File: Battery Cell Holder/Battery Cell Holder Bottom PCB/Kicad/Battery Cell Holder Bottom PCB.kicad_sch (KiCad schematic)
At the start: 10 parts

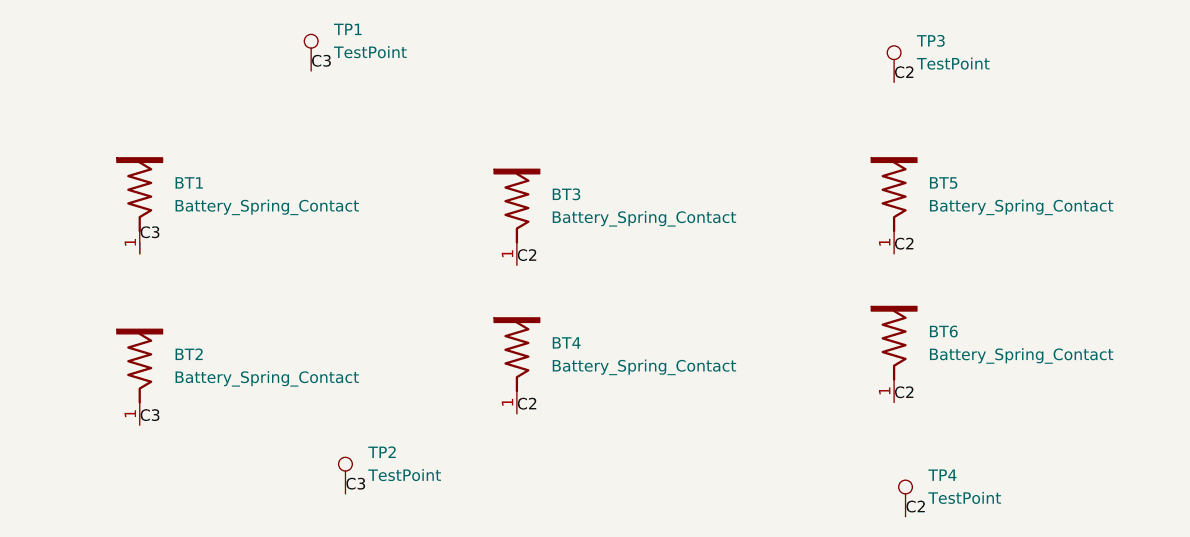
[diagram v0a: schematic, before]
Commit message: fixes to boards
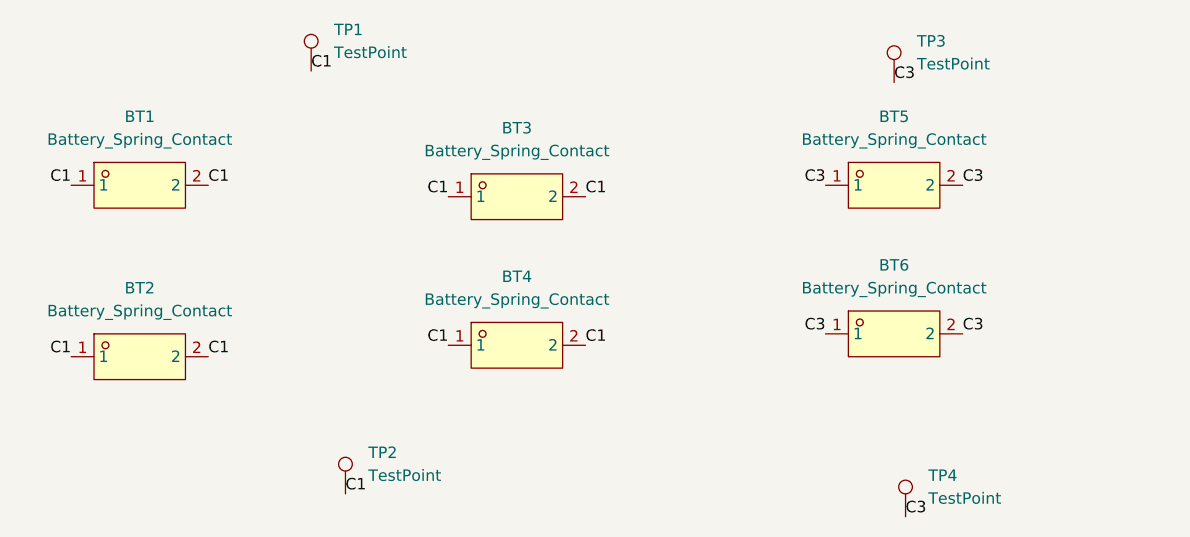
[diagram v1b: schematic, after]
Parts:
- BT1, BT2, BT3, BT4, BT5, BT6: footprint BatterySpringContact:Keystone_5222_SpringContact_THM -> C19724688:TH-2_BD10.0_F10-12-0.5-1.3UU-SUS304; symbol BatterySpringContact:Battery_Spring_Contact -> C19724688:F10-12-0.5-1.3UU-SUS304; LCSC Part (none) -> C19724688; MPN (none) -> F10-12-0.5-1.3UU-sus304; Manufacturer (none) -> XMXW(芯网)
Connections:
- net C3: now also BT5.1, BT5.2, BT6.1, BT6.2, TP3.1, TP4.1; no longer BT1.1, BT2.1, TP1.1, TP2.1
- removed net C2: BT3.1, BT4.1, BT5.1, BT6.1, TP3.1, TP4.1
- new net C1: BT1.1, BT1.2, BT2.1, BT2.2, BT3.1, BT3.2, BT4.1, BT4.2, TP1.1, TP2.1
